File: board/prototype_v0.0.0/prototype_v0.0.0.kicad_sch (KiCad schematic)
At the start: 6 parts, among them U1 ATmega328PB-A, U2 CH340C, Y1 16MHz

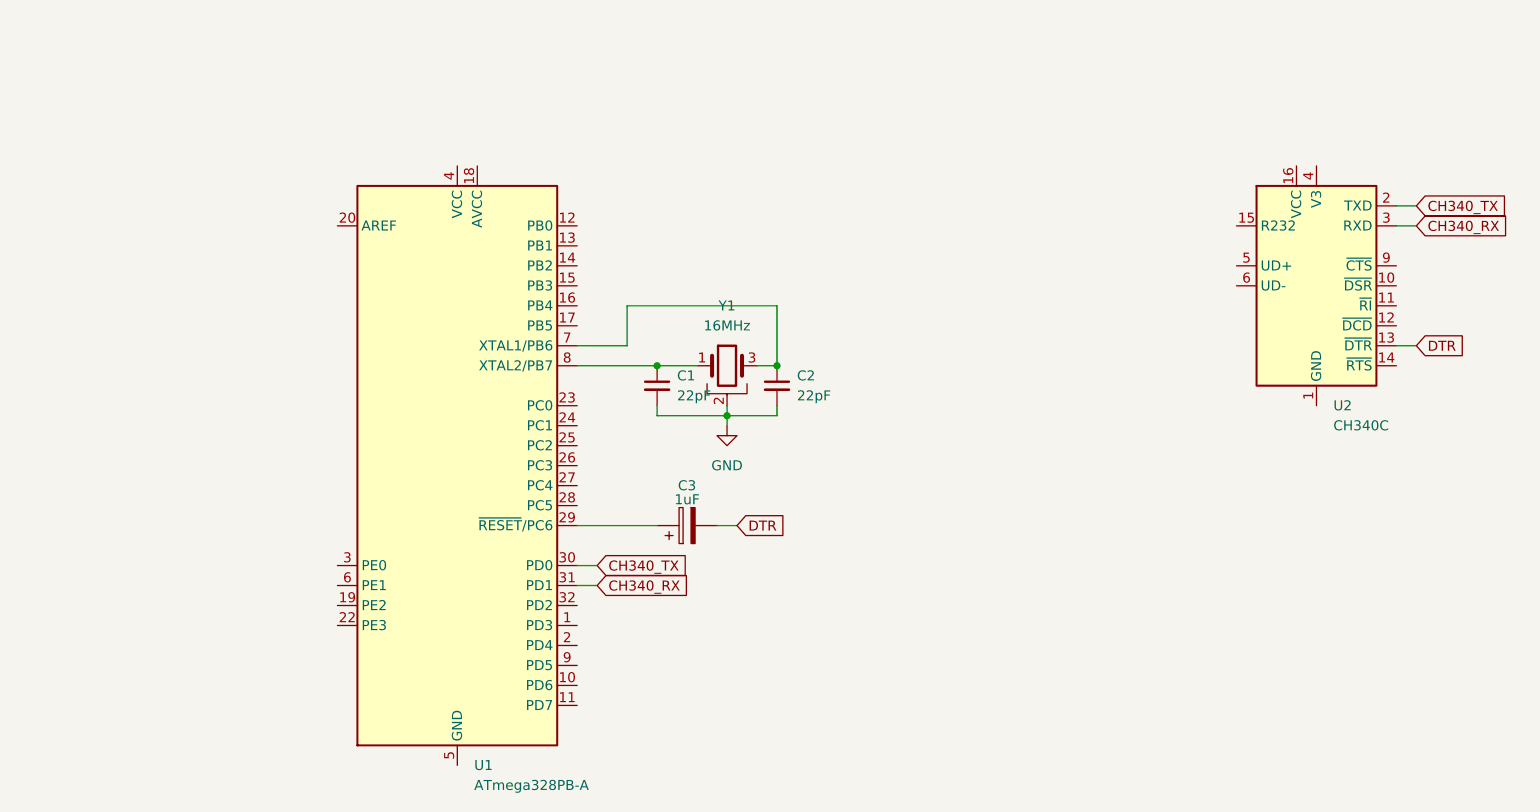
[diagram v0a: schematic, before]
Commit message: BRD schematic update
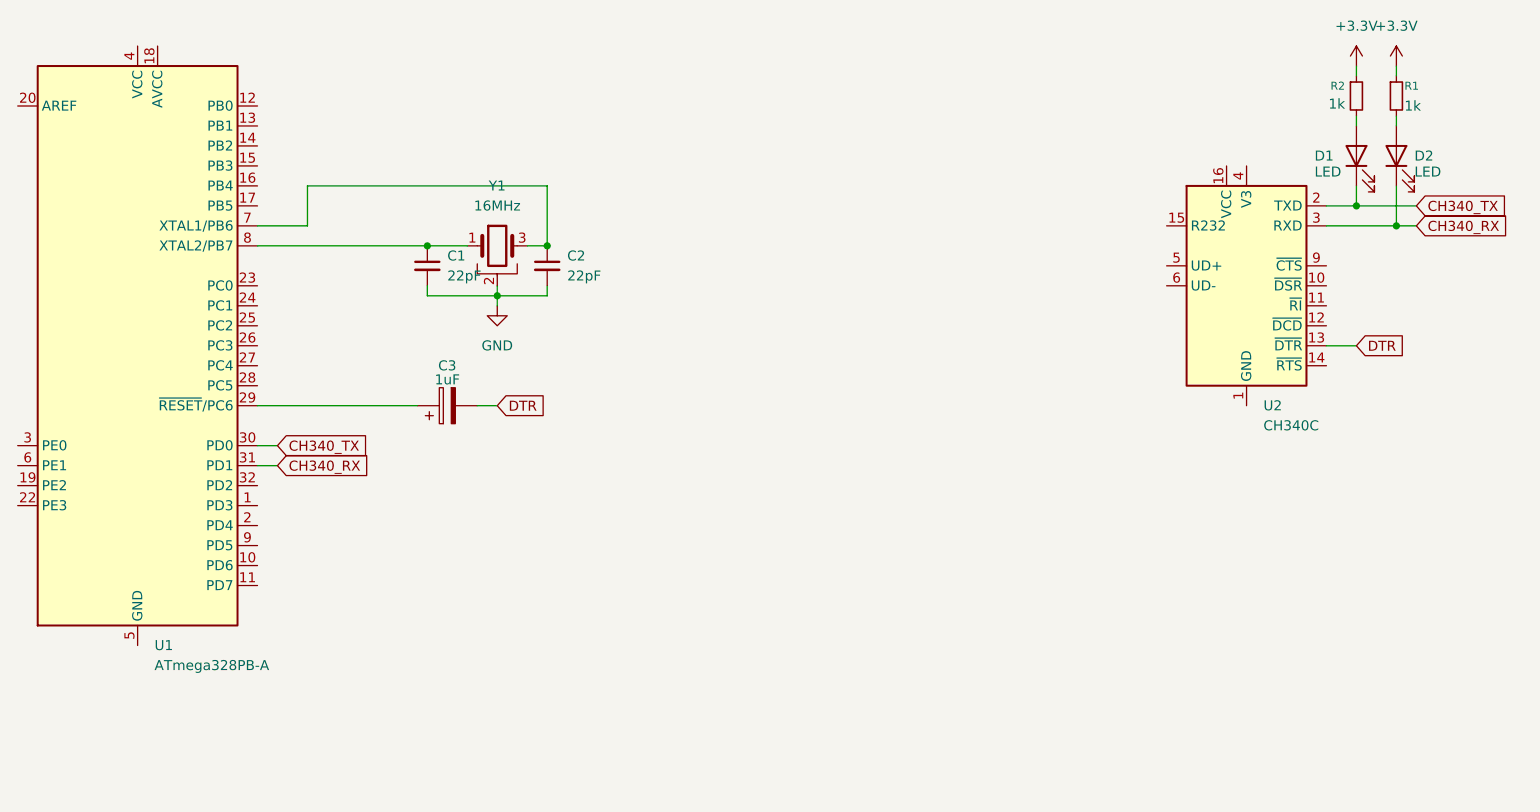
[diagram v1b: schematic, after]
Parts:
- added D1, D2: LED, symbol Device:LED
- added R1, R2: 1k, symbol Device:R_Small
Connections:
- net CH340_RX: now also D2.1 (K)
- net CH340_TX: now also D1.1 (K)
- new net: D2.2 (A), R1.2
- new net: D1.2 (A), R2.2
- new net +3.3V: R1.1, R2.1
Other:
- moved on the sheet: C1, C2, C3, U1, U2, Y1
